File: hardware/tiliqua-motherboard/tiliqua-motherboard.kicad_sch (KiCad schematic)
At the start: 27 parts, among them J2 Conn_02x06_Top_Bottom, J3 Conn_02x06_Top_Bottom, J8 MICROMOD-2222, U11 Si5351A-B-GT, U6 74AUC1G79, Y2 25MHz AMB8G

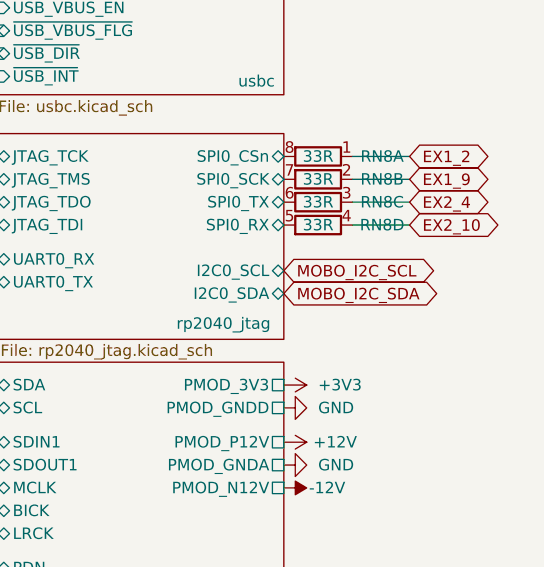
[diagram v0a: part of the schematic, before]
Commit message: * fab 05.01.24
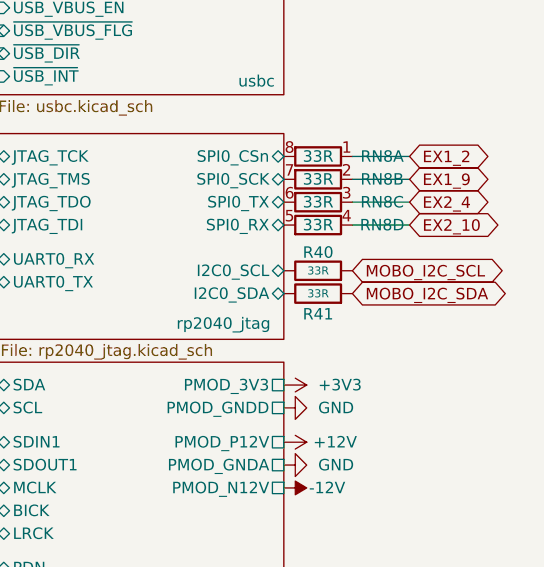
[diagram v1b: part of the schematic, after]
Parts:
- added R40, R41: 33R, Resistor_SMD:R_0402_1005Metric, symbol OLIMEX_RCL:R
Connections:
- net MOBO_I2C_SCL: now also R40.2
- net MOBO_I2C_SDA: now also R41.2
- new net rp2040_jtag/I2C0_SCL: R40.1
- new net rp2040_jtag/I2C0_SDA: R41.1
